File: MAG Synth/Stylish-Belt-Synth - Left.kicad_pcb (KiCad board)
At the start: 2 copper layers, 88.9 x 101.7 mm, 18 parts, among them J26 WRITE PATCH, J27 PARAM SELECT, J28 PATCH SELECT, J29 MODE, U1 stm32f103c8t6-module-china_smd

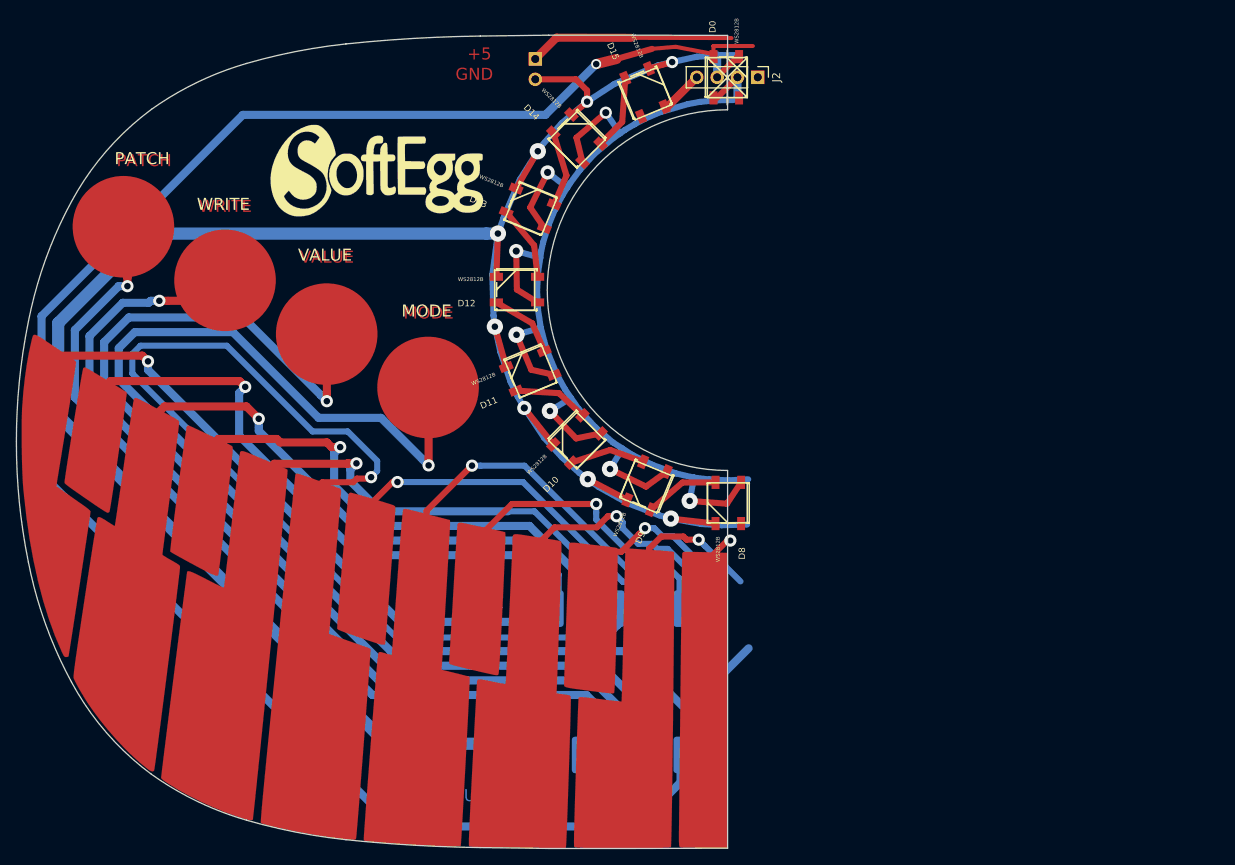
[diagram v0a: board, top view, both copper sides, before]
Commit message: Latest
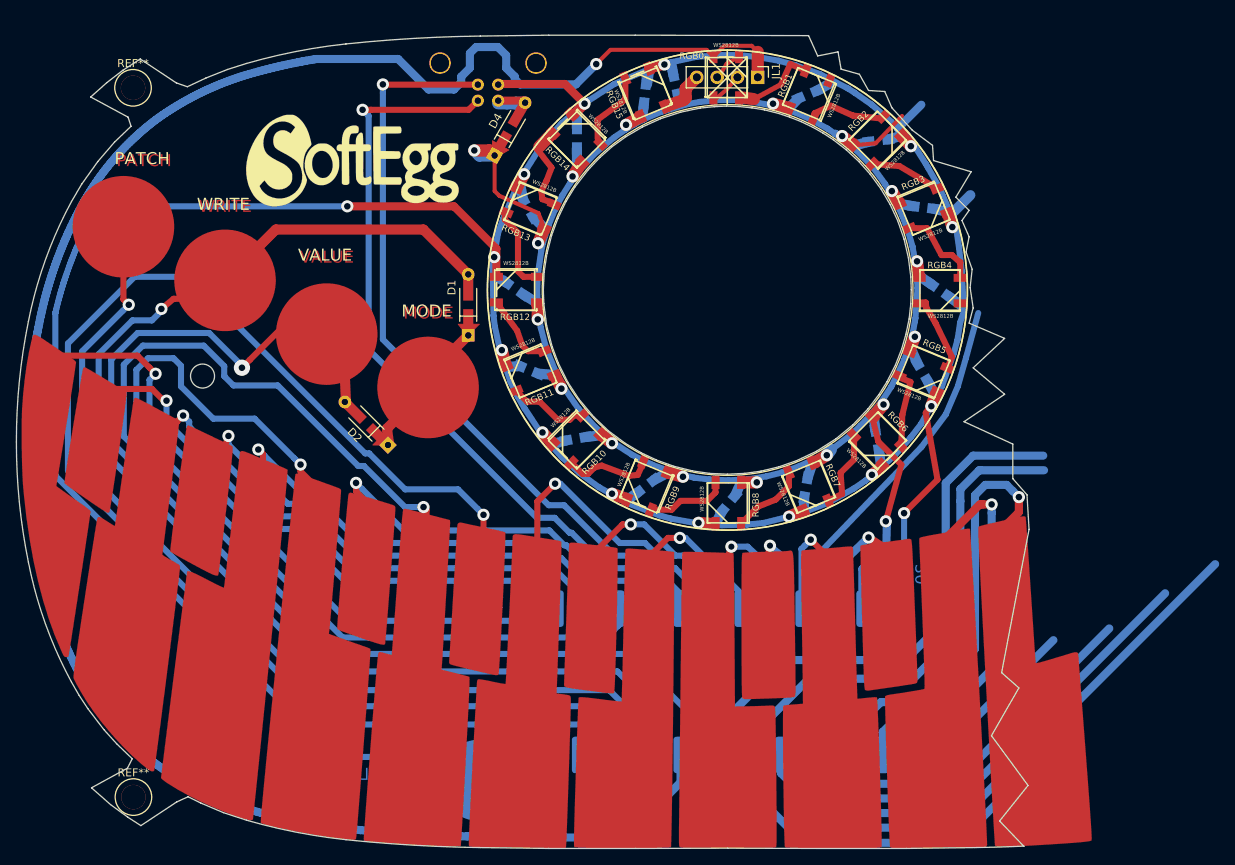
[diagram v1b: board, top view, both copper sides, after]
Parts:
- removed BT1: 4 x 1.5V, Pin_Headers:Pin_Header_Angled_1x02_Pitch2.54mm
- removed D15: WS2812B, WS2812B
- removed J2: ~, Pin_Headers:Pin_Header_Straight_1x04_Pitch2.54mm
- added CL0: 104, Capacitors_SMD:C_0805_HandSoldering, B.Cu at (142.0, 60.4)
- added CL1: 104, Capacitors_SMD:C_0805_HandSoldering, B.Cu at (158.5, 61.6)
- added CL10: 104, Capacitors_SMD:C_0805_HandSoldering, B.Cu at (129.5, 104.6)
- added CL11: 104, Capacitors_SMD:C_0805_HandSoldering, B.Cu at (123.7, 96.0)
- added CL12: 104, Capacitors_SMD:C_0805_HandSoldering, B.Cu at (121.9, 85.9)
- added CL13: 104, Capacitors_SMD:C_0805_HandSoldering, B.Cu at (123.6, 75.8)
- added CL14: 104, Capacitors_SMD:C_0805_HandSoldering, B.Cu at (129.7, 67.1)
- added CL15: 104, Capacitors_SMD:C_0805_HandSoldering, B.Cu at (138.2, 61.5)
- added CL2: 104, Capacitors_SMD:C_0805_HandSoldering, B.Cu at (167.4, 67.3)
- added CL3: 104, Capacitors_SMD:C_0805_HandSoldering, B.Cu at (173.0, 75.7)
- added CL4: 104, Capacitors_SMD:C_0805_HandSoldering, B.Cu at (175.1, 86.1)
- added CL5: 104, Capacitors_SMD:C_0805_HandSoldering, B.Cu at (172.9, 96.3)
- added CL6: 104, Capacitors_SMD:C_0805_HandSoldering, B.Cu at (167.2, 104.8)
- added CL7: 104, Capacitors_SMD:C_0805_HandSoldering, B.Cu at (158.3, 110.7)
- added CL8: 104, Capacitors_SMD:C_0805_HandSoldering, B.Cu at (148.6, 112.7)
- added CL9: 104, Capacitors_SMD:C_0805_HandSoldering, B.Cu at (138.3, 110.5)
- added D1: 1N4148, SoftEggKiCAD:D_DO-35_SOD27_P7.62mm_Horizontal+SMD, F.Cu at (116.1, 91.7)
- added D2: 1N4148, SoftEggKiCAD:D_DO-35_SOD27_P7.62mm_Horizontal+SMD, F.Cu at (106.0, 105.4)
- added D4: 1N5822, SoftEggKiCAD:D_DO-35_SOD27_P7.62mm_Horizontal+SMD, F.Cu at (119.4, 69.2)
- added J0: USB_B, Connectors:USB_B, B.Cu at (119.8, 62.4)
- added J30: STYLUS, SoftEggKiCAD:LargeRoundTouchPad, B.Cu at (117.5, 147.3)
- added JL1: ~, Pin_Headers:Pin_Header_Straight_1x04_Pitch2.54mm, F.Cu at (152.3, 59.4)
- added REF**: AA Battery Holder, SoftEggKiCAD:AA_Battery_Holder_SoftEgg, B.Cu at (82.9, 104.6)
- added REF**: 1pin, Connect:1pin, F.Cu at (74.2, 60.8)
- added REF**: 1pin, Connect:1pin, F.Cu at (74.2, 149.4)
- added RGB1: WS2812B, WS2812B:WS2812B, F.Cu at (158.8, 61.6)
- added RGB15: WS2812B, WS2812B:WS2812B, F.Cu at (138.2, 61.3)
- added RGB2: WS2812B, WS2812B:WS2812B, F.Cu at (167.3, 67.3)
- added RGB3: WS2812B, WS2812B:WS2812B, F.Cu at (173.0, 75.8)
- added RGB4: WS2812B, WS2812B:WS2812B, F.Cu at (175.0, 86.1)
- added RGB5: WS2812B, WS2812B:WS2812B, F.Cu at (173.0, 96.3)
- added RGB6: WS2812B, WS2812B:WS2812B, F.Cu at (167.3, 104.9)
- added RGB7: WS2812B, WS2812B:WS2812B, F.Cu at (158.6, 110.6)
- KB1: footprint SoftEggKiCAD:MAGWestSynthContactKeybedLeft -> SoftEggKiCAD:MAGWestSynthContactKeybed
- RGB0: renamed from D0; footprint WS2812B -> WS2812B:WS2812B
- RGB10: renamed from D10; footprint WS2812B -> WS2812B:WS2812B
- RGB11: renamed from D11; footprint WS2812B -> WS2812B:WS2812B
- RGB12: renamed from D12; footprint WS2812B -> WS2812B:WS2812B
- RGB13: renamed from D13; footprint WS2812B -> WS2812B:WS2812B
- RGB14: renamed from D14; footprint WS2812B -> WS2812B:WS2812B
- RGB8: renamed from D8; footprint WS2812B -> WS2812B:WS2812B
- RGB9: renamed from D9; footprint WS2812B -> WS2812B:WS2812B
- U1: value stm32f103c8t6-module-china_smd -> stm32f103c8t6-module-china
- moved G*** 3.30 mm to (101.6, 69.8)
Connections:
- J26 pad 1: Net-(J26-Pad1) -> /WRITE
- J27 pad 1: Net-(J27-Pad1) -> /PARAM
- J28 pad 1: Net-(J28-Pad1) -> /PATCH
- KB1 pad 0: Net-(KB1-Pad0) -> /C0
- KB1 pad 1: Net-(KB1-Pad1) -> /C#0
- KB1 pad 10: Net-(KB1-Pad10) -> /A#0
- KB1 pad 11: Net-(KB1-Pad11) -> /B0
- KB1 pad 12: Net-(KB1-Pad12) -> /C1
- KB1 pad 2: Net-(KB1-Pad2) -> /D0
- KB1 pad 3: Net-(KB1-Pad3) -> /D#0
- KB1 pad 4: Net-(KB1-Pad4) -> /E0
- KB1 pad 5: Net-(KB1-Pad5) -> /F0
- KB1 pad 6: Net-(KB1-Pad6) -> /F#0
- KB1 pad 7: Net-(KB1-Pad7) -> /G0
- KB1 pad 8: Net-(KB1-Pad8) -> /G#0
- KB1 pad 9: Net-(KB1-Pad9) -> /A0
- RGB0 pad 1: /WS2812B-16-LED-RING/5V -> /+5V
- RGB0 pad 3: /WS2812B-16-LED-RING/GND -> GND
- RGB0 pad 4: /WS2812B-16-LED-RING/DIN -> /LED_DIN
- RGB10 pad 1: /WS2812B-16-LED-RING/5V -> /+5V
- RGB10 pad 3: /WS2812B-16-LED-RING/GND -> GND
- RGB11 pad 1: /WS2812B-16-LED-RING/5V -> /+5V
- RGB11 pad 3: /WS2812B-16-LED-RING/GND -> GND
- RGB12 pad 1: /WS2812B-16-LED-RING/5V -> /+5V
- RGB12 pad 3: /WS2812B-16-LED-RING/GND -> GND
- RGB13 pad 1: /WS2812B-16-LED-RING/5V -> /+5V
- RGB13 pad 3: /WS2812B-16-LED-RING/GND -> GND
- RGB14 pad 1: /WS2812B-16-LED-RING/5V -> /+5V
- RGB14 pad 3: /WS2812B-16-LED-RING/GND -> GND
- RGB8 pad 1: /WS2812B-16-LED-RING/5V -> /+5V
- RGB8 pad 3: /WS2812B-16-LED-RING/GND -> GND
- RGB9 pad 1: /WS2812B-16-LED-RING/5V -> /+5V
- RGB9 pad 3: /WS2812B-16-LED-RING/GND -> GND
- U1 pad 1: (no net) -> /C0
- U1 pad 10: (no net) -> /A0
- U1 pad 11: (no net) -> /A#0
- U1 pad 2: (no net) -> /C#0
- U1 pad 3: (no net) -> /D0
- U1 pad 30: (no net) -> /C2
- U1 pad 31: (no net) -> /G0
- U1 pad 32: (no net) -> /LED_DIN
- U1 pad 33: (no net) -> /PARAM
- U1 pad 34: (no net) -> /WRITE
- U1 pad 35: (no net) -> /PATCH
- U1 pad 36: (no net) -> /G#0
- U1 pad 37: (no net) -> Net-(U1-Pad37)
- U1 pad 38: (no net) -> Net-(U1-Pad38)
- U1 pad 39: (no net) -> GND
- U1 pad 4: (no net) -> /D#0
- U1 pad 40: (no net) -> GND
- U1 pad 5: (no net) -> /E0
- U1 pad 6: (no net) -> /F0
- U1 pad 7: (no net) -> /F#0
- U1 pad 8: (no net) -> Net-(J0-Pad2)
- U1 pad 9: (no net) -> Net-(J0-Pad3)
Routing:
- net GND: track 0.00 -> 457.8 mm, vias 0 -> 15
- net /WS2812B-16-LED-RING/GND: track 296.0 -> 0.00 mm, vias 8 -> 0
- net /+5V: track 0.00 -> 267.1 mm, vias 0 -> 17
- net /LED_DIN: track 0.00 -> 256.1 mm, vias 0 -> 1
- net /WS2812B-16-LED-RING/DIN: track 228.9 -> 0.00 mm, vias 1 -> 0
- net /G#0: track 0.00 -> 166.6 mm, vias 0 -> 1
- net /WS2812B-16-LED-RING/5V: track 161.7 -> 0.00 mm, vias 7 -> 0
- net /WRITE: track 0.00 -> 151.2 mm, vias 0 -> 1
- net /G0: track 0.00 -> 147.7 mm, vias 0 -> 1
- net /PARAM: track 0.00 -> 142.8 mm, vias 0 -> 1
- net Net-(J27-Pad1): track 136.7 -> 0.00 mm, vias 1 -> 0
- net Net-(D1-Pad1): track 153.1 -> 17.7 mm, vias 1 -> 0
- net Net-(KB1-Pad5): track 124.6 -> 0.00 mm, vias 1 -> 0
- net /PATCH: track 0.00 -> 115.1 mm, vias 0 -> 1
- net Net-(J26-Pad1): track 114.9 -> 0.00 mm, vias 1 -> 0
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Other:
- board size 88.9 x 101.7 mm -> 126.6 x 101.7 mm
- net class Default: trace_width 0.508 -> 0.2
- board text added: "20"
- board text added: "Stylish!"
- board text removed: "+5"
- board text removed: "GND"
